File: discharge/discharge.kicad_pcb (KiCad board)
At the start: 2 copper layers, 84 x 45 mm, 16 parts, among them J1 Conn_SDC, J2 Conn_HV_IN, J3 Conn_HV_OUT, J4 GND, J5 Conn_HV_IN, J6 Conn_HV_OUT, K1 Relay_SPST-NC, K2 Relay_SPST-NC

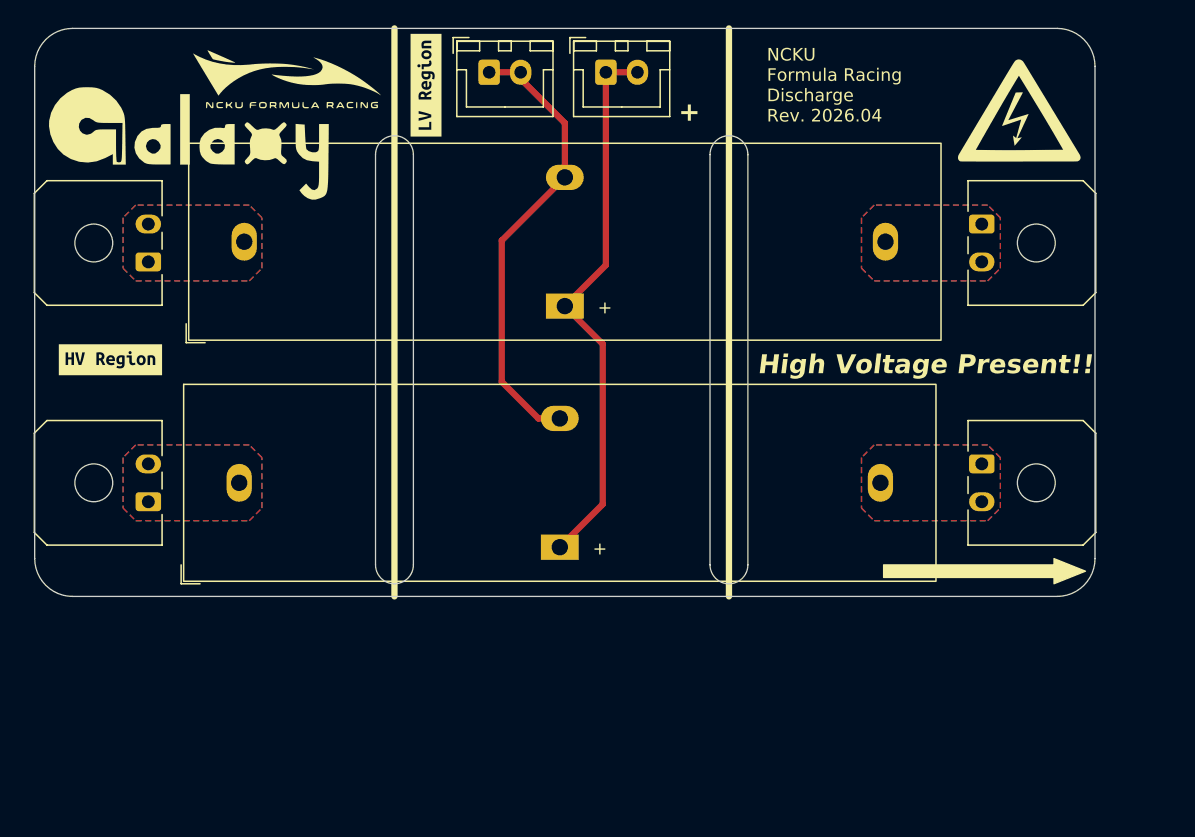
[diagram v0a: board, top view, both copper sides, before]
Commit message: finish timer layout
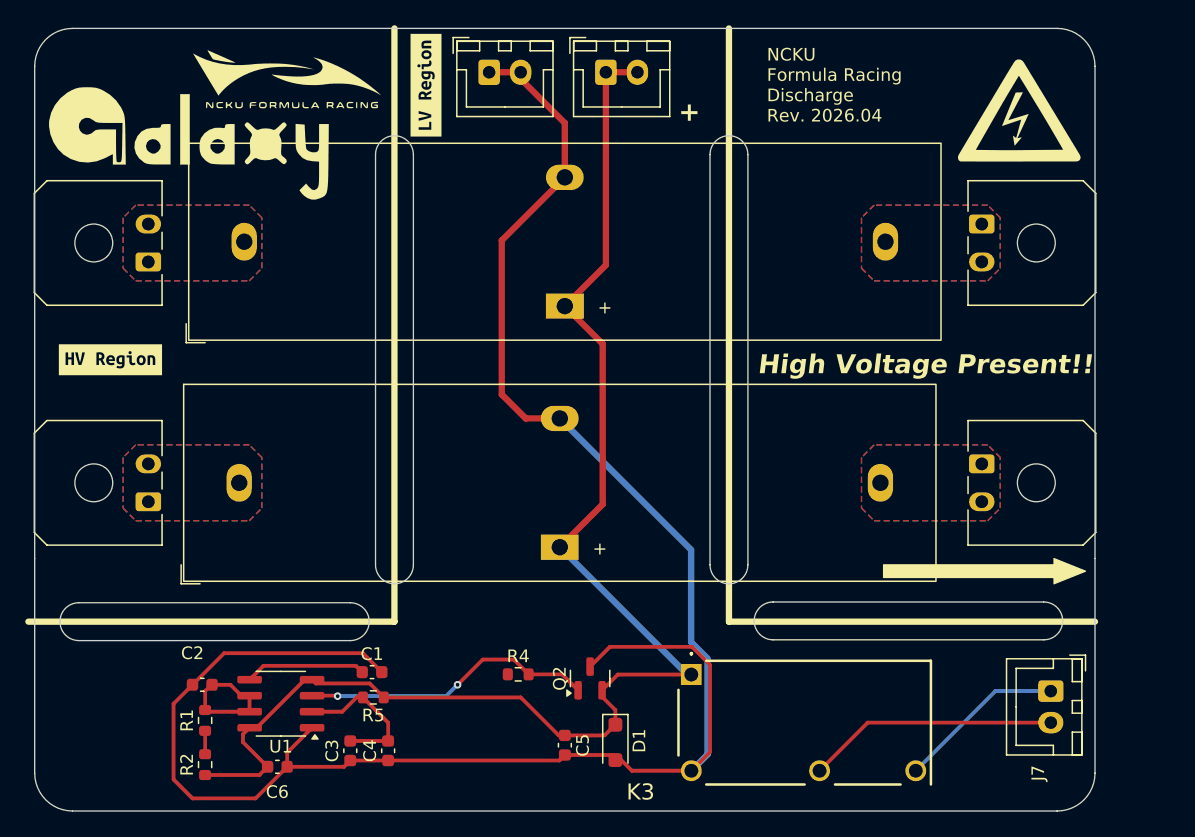
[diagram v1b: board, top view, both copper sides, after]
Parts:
- added C1: 100n, Capacitor_SMD:C_0603_1608Metric, F.Cu at (116.7, 120.0)
- added C2: 100u, Capacitor_SMD:C_0603_1608Metric, F.Cu at (103.3, 121.0)
- added C3: 100n, Capacitor_SMD:C_0603_1608Metric, F.Cu at (115.0, 126.2)
- added C4: 100n, Capacitor_SMD:C_0603_1608Metric, F.Cu at (118.0, 126.2)
- added C5: 1u, Capacitor_SMD:C_0603_1608Metric, F.Cu at (132.0, 125.8)
- added C6: 1u, Capacitor_SMD:C_0603_1608Metric, F.Cu at (109.2, 127.5)
- added D1: D_Small, Diode_SMD:D_SOD-123F, F.Cu at (136.0, 125.6)
- added J7: Conn, Connector_JST:JST_XH_B2B-XH-A_1x02_P2.50mm_Vertical, F.Cu at (170.5, 121.5)
- added K3: JY-12H-K, JY12Hk:JY12HK, F.Cu at (142.0, 120.2)
- added Q2: Si2301CDS, Package_TO_SOT_SMD:SOT-23, F.Cu at (134.0, 120.5)
- added R1: 4.7k, Resistor_SMD:R_0603_1608Metric, F.Cu at (103.5, 123.8)
- added R2: 68k, Resistor_SMD:R_0603_1608Metric, F.Cu at (103.5, 127.3)
- added R4: 10k, Resistor_SMD:R_0603_1608Metric, F.Cu at (128.3, 120.2)
- added R5: 10k, Resistor_SMD:R_0603_1608Metric, F.Cu at (116.8, 122.0)
- added U1: SE555D, Package_SO:SOIC-8_3.9x4.9mm_P1.27mm, F.Cu at (109.5, 122.5)
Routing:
- net GND: track 36.3 -> 162.2 mm
- net VDC: track 44.1 -> 111.5 mm
- net Timer: track 0.00 -> 23.3 mm, vias 0 -> 2
- net Net-(J7-Pin_2): track 0.00 -> 19.9 mm
- net Net-(J7-Pin_1): track 0.00 -> 13.3 mm
- net Net-(U1-TR): track 0.00 -> 11.8 mm
- net Net-(U1-DIS): track 0.00 -> 10.4 mm
- net Net-(U1-CV): track 0.00 -> 9.59 mm
- net Net-(R1-Pad1): track 0.00 -> 1.85 mm
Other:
- board size 84 x 45 mm -> 84 x 62 mm
